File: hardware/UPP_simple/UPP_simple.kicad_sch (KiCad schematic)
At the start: 9 parts, among them IC2 STM32G0C1KCT6N

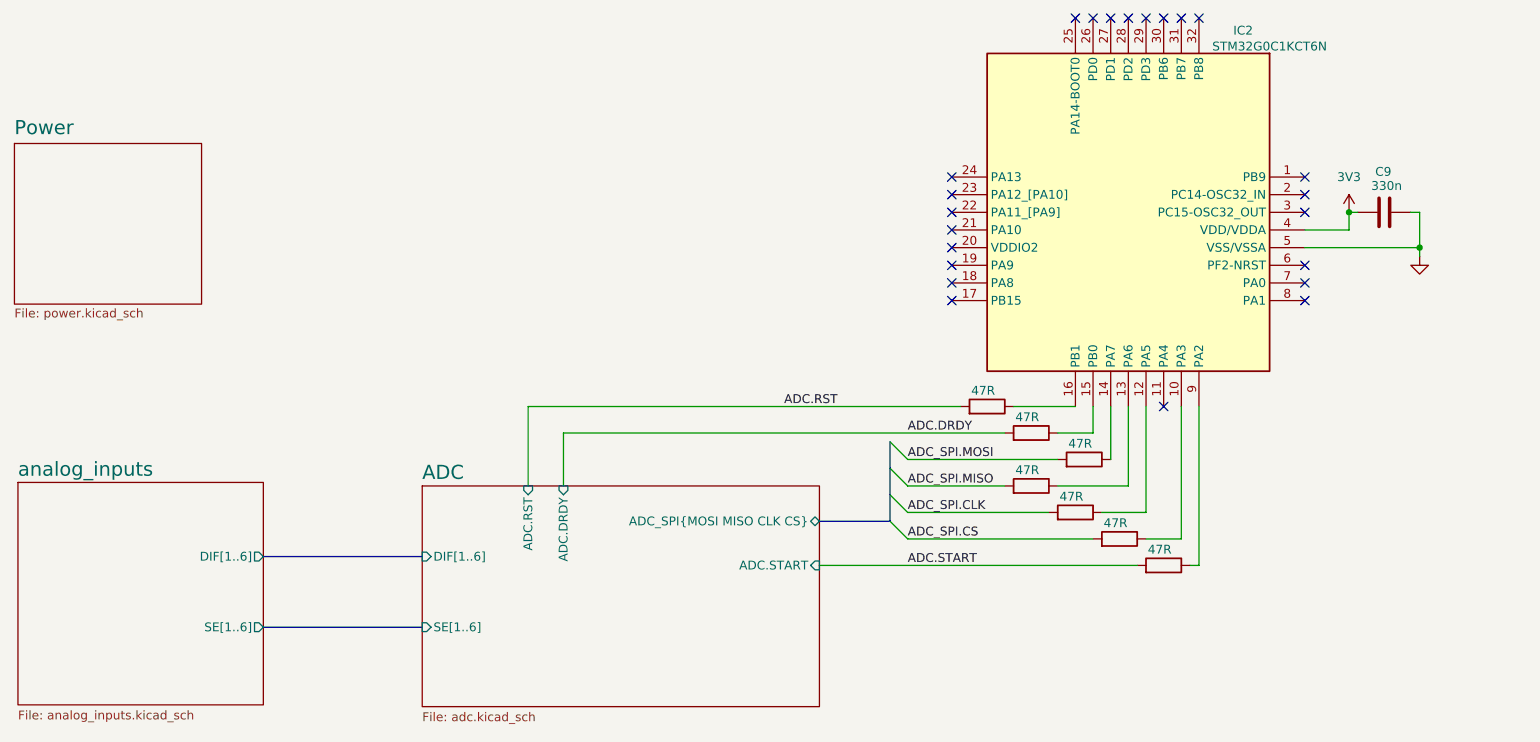
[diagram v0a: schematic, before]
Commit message: Add files via upload
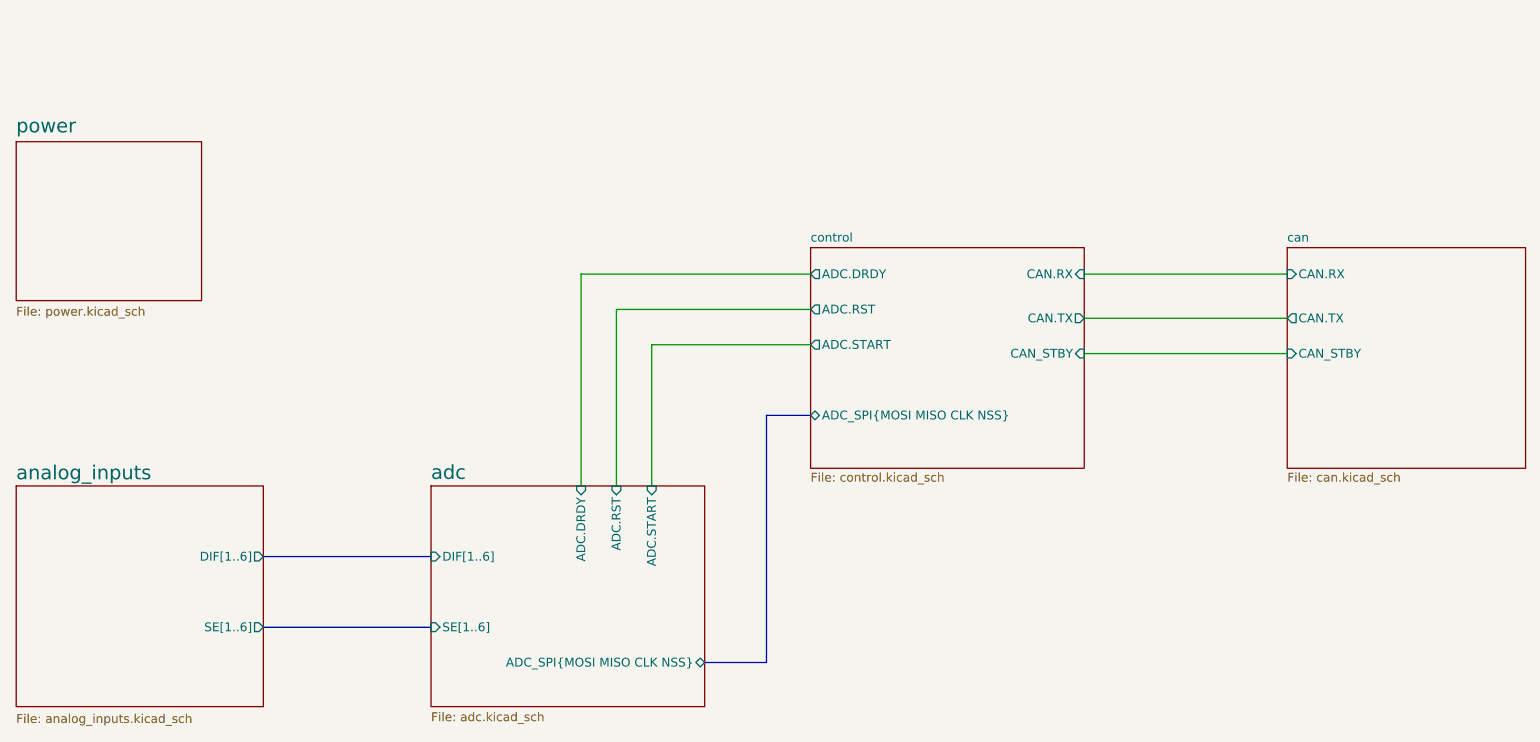
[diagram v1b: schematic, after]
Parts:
- removed C9: 330n, Capacitor_SMD:C_0603_1608Metric_Pad1.08x0.95mm_HandSolder, symbol Device:C
- removed IC2: STM32G0C1KCT6N, QFP80P900X900X160-32N, symbol STM32G0C1KCT6N:STM32G0C1KCT6N
- removed R10, R11, R12, R13, R14, R15, R9: 47R, Resistor_SMD:R_0603_1608Metric_Pad0.98x0.95mm_HandSolder, symbol Device:R
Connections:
- no-connect marks 23 -> 0
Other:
- sheet ADC renamed adc
- sheet Power renamed power
- added sheet can (can.kicad_sch)
- added sheet control (control.kicad_sch)
- sheet adc ports: added ADC_SPI{MOSI MISO CLK NSS}; removed ADC_SPI{MOSI MISO CLK CS}
